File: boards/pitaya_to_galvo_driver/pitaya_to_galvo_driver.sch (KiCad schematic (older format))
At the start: 2 parts

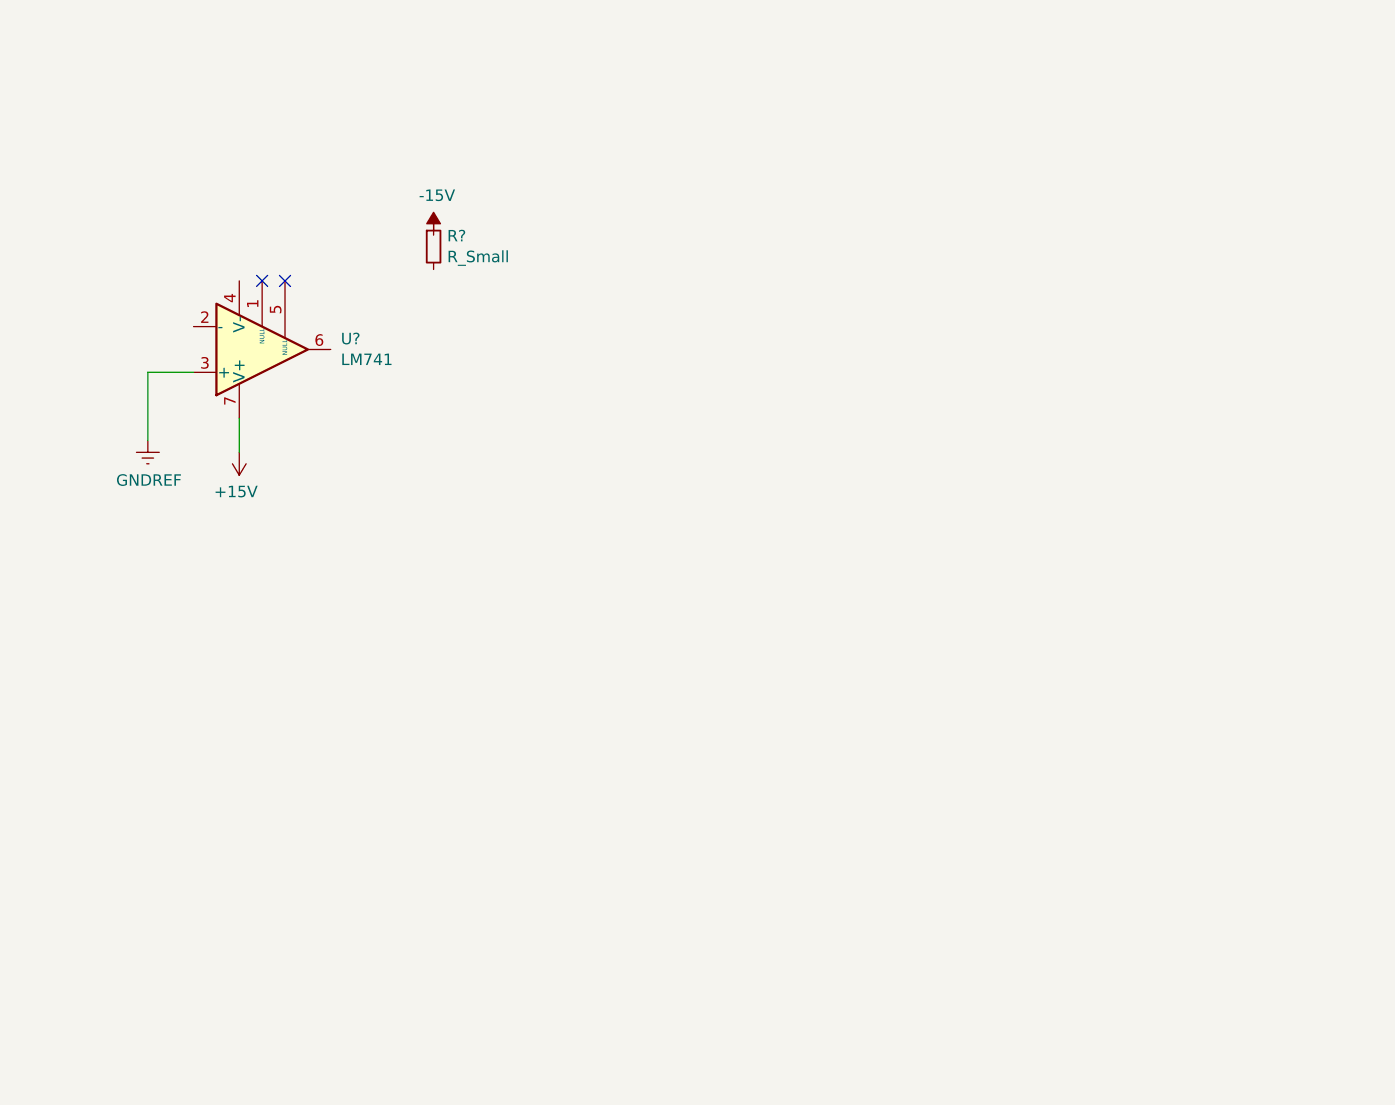
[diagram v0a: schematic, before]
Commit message: first stage of the board
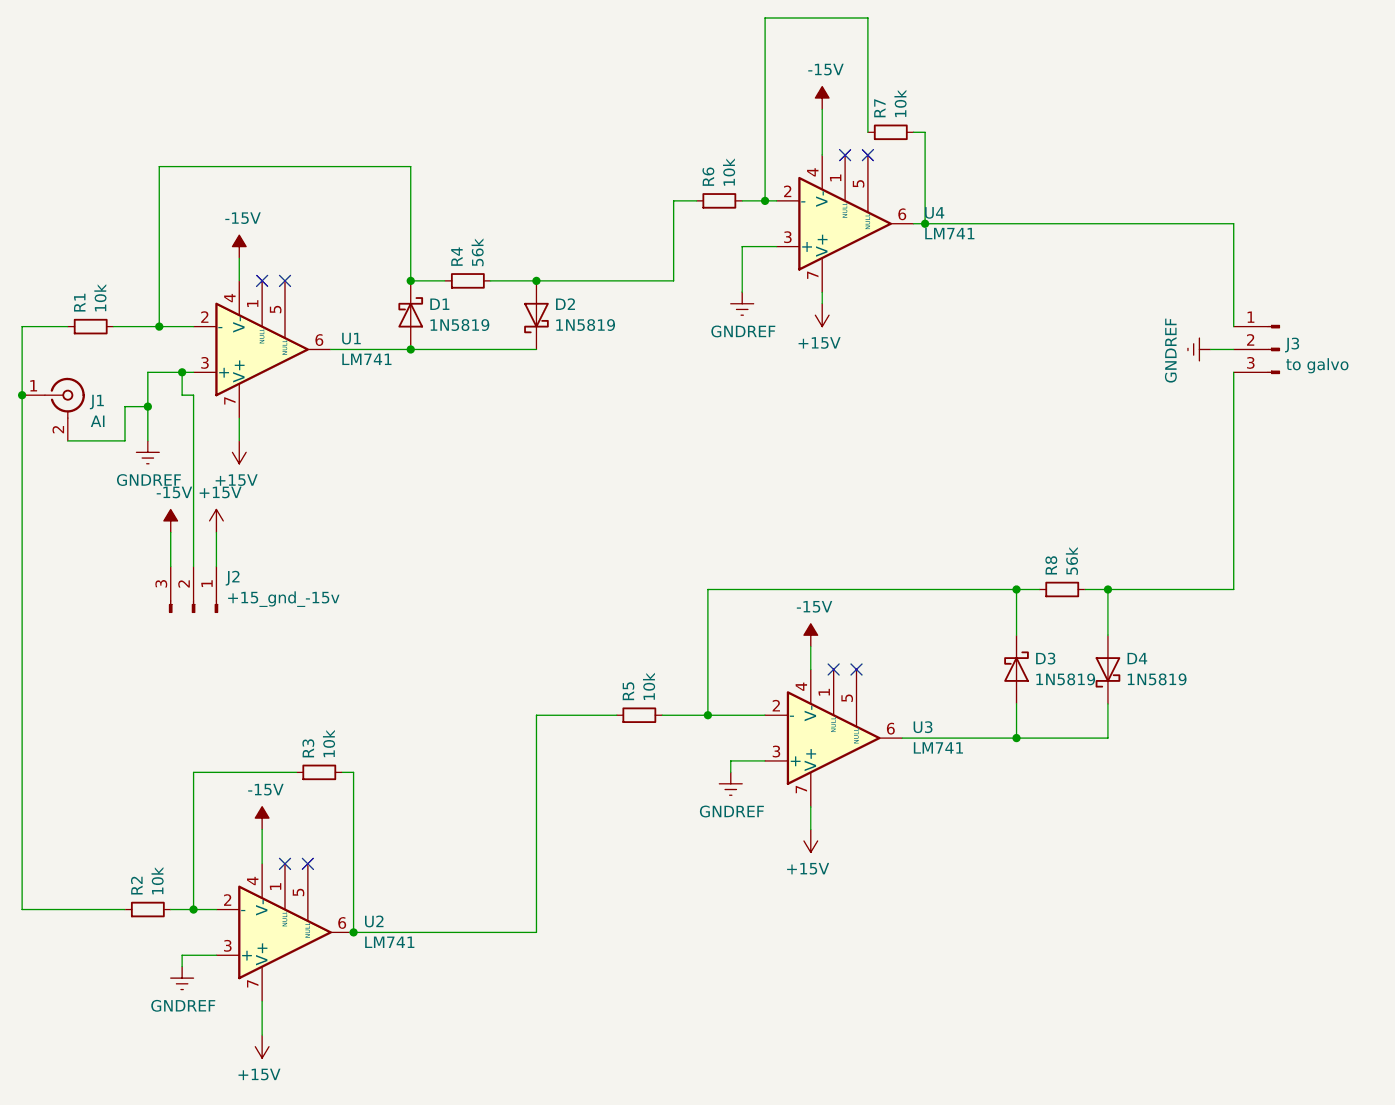
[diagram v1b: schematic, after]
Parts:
- added D1, D2, D3, D4: 1N5819, Diode_THT:D_DO-41_SOD81_P10.16mm_Horizontal, symbol Diode:1N5819
- added J1: AI, Connector_Coaxial:BNC_Amphenol_B6252HB-NPP3G-50_Horizontal, symbol Connector:Conn_Coaxial
- added J2: +15_gnd_-15v, Connector_JST:JST_XH_B3B-XH-A_1x03_P2.50mm_Vertical, symbol Connector:Conn_01x03_Male
- added J3: to galvo, Connector_JST:JST_XH_B3B-XH-A_1x03_P2.50mm_Vertical, symbol Connector:Conn_01x03_Male
- added R2, R3, R5, R6, R7: 10k, Resistor_THT:R_Axial_DIN0207_L6.3mm_D2.5mm_P10.16mm_Horizontal, symbol Device:R_Small
- added R4, R8: 56k, Resistor_THT:R_Axial_DIN0207_L6.3mm_D2.5mm_P10.16mm_Horizontal, symbol Device:R_Small
- added U2, U3, U4: LM741, Package_DIP:DIP-8_W7.62mm_Socket, symbol Amplifier_Operational:LM741
- R1: renamed from R?; value R_Small -> 10k; footprint (none) -> Resistor_THT:R_Axial_DIN0207_L6.3mm_D2.5mm_P10.16mm_Horizontal
- U1: renamed from U?; footprint (none) -> Package_DIP:DIP-8_W7.62mm_Socket
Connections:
- net +15V: now also J2.1 (Pin_1), U2.7 (V+), U3.7 (V+), U4.7 (V+)
- net -15V: now also U1.4 (V-), J2.3 (Pin_3), U2.4 (V-), U3.4 (V-), U4.4 (V-)
- net GNDREF: now also J1.2 (Ext), J2.2 (Pin_2), J3.2 (Pin_2), U2.3 (+), U3.3 (+), U4.3 (+)
- net at U1.2 (-): now also R1.2, D1.1 (K), R4.1
- net at U1.6: now also D1.2 (A), D2.1 (K)
- net at R1.1: now also J1.1 (In), R2.1
- new net: D2.2 (A), R4.2, R6.1
- new net: R6.2, R7.1, U4.2 (-)
- new net: J3.1 (Pin_1), R7.2, U4.6
- new net: R2.2, R3.1, U2.2 (-)
- new net: R3.2, R5.1, U2.6
- new net: D3.1 (K), R5.2, R8.1, U3.2 (-)
- new net: D3.2 (A), D4.1 (K), U3.6
- new net: D4.2 (A), J3.3 (Pin_3), R8.2
- no-connect marks 2 -> 8
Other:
- moved on the sheet: R1
